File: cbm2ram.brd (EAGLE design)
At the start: 133.3 x 120.7 mm, 21 parts, among them U1 74574N, U2 74574N, U3 GAL16V8, U4 74LS04N, U5 HM628512A_DIL32, U6 HM628512A_DIL32, U7 74541N, U8 74541N

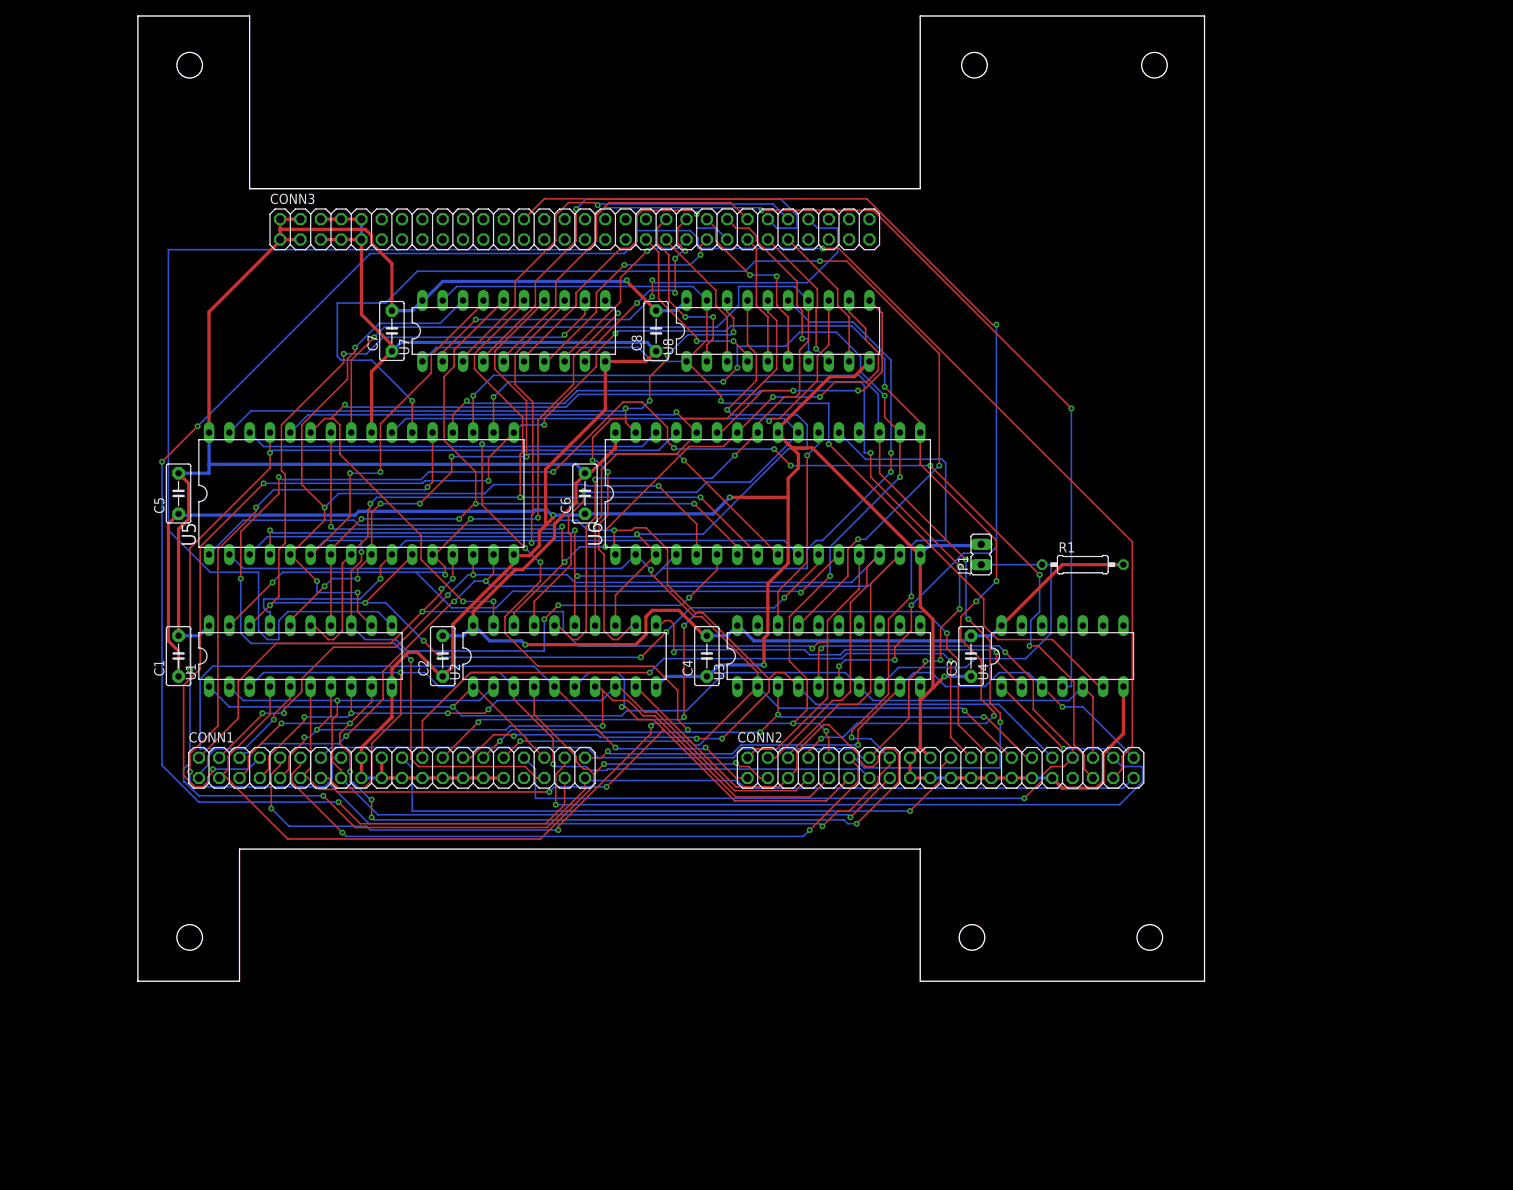
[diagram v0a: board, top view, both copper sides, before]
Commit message: Added EPROM chips
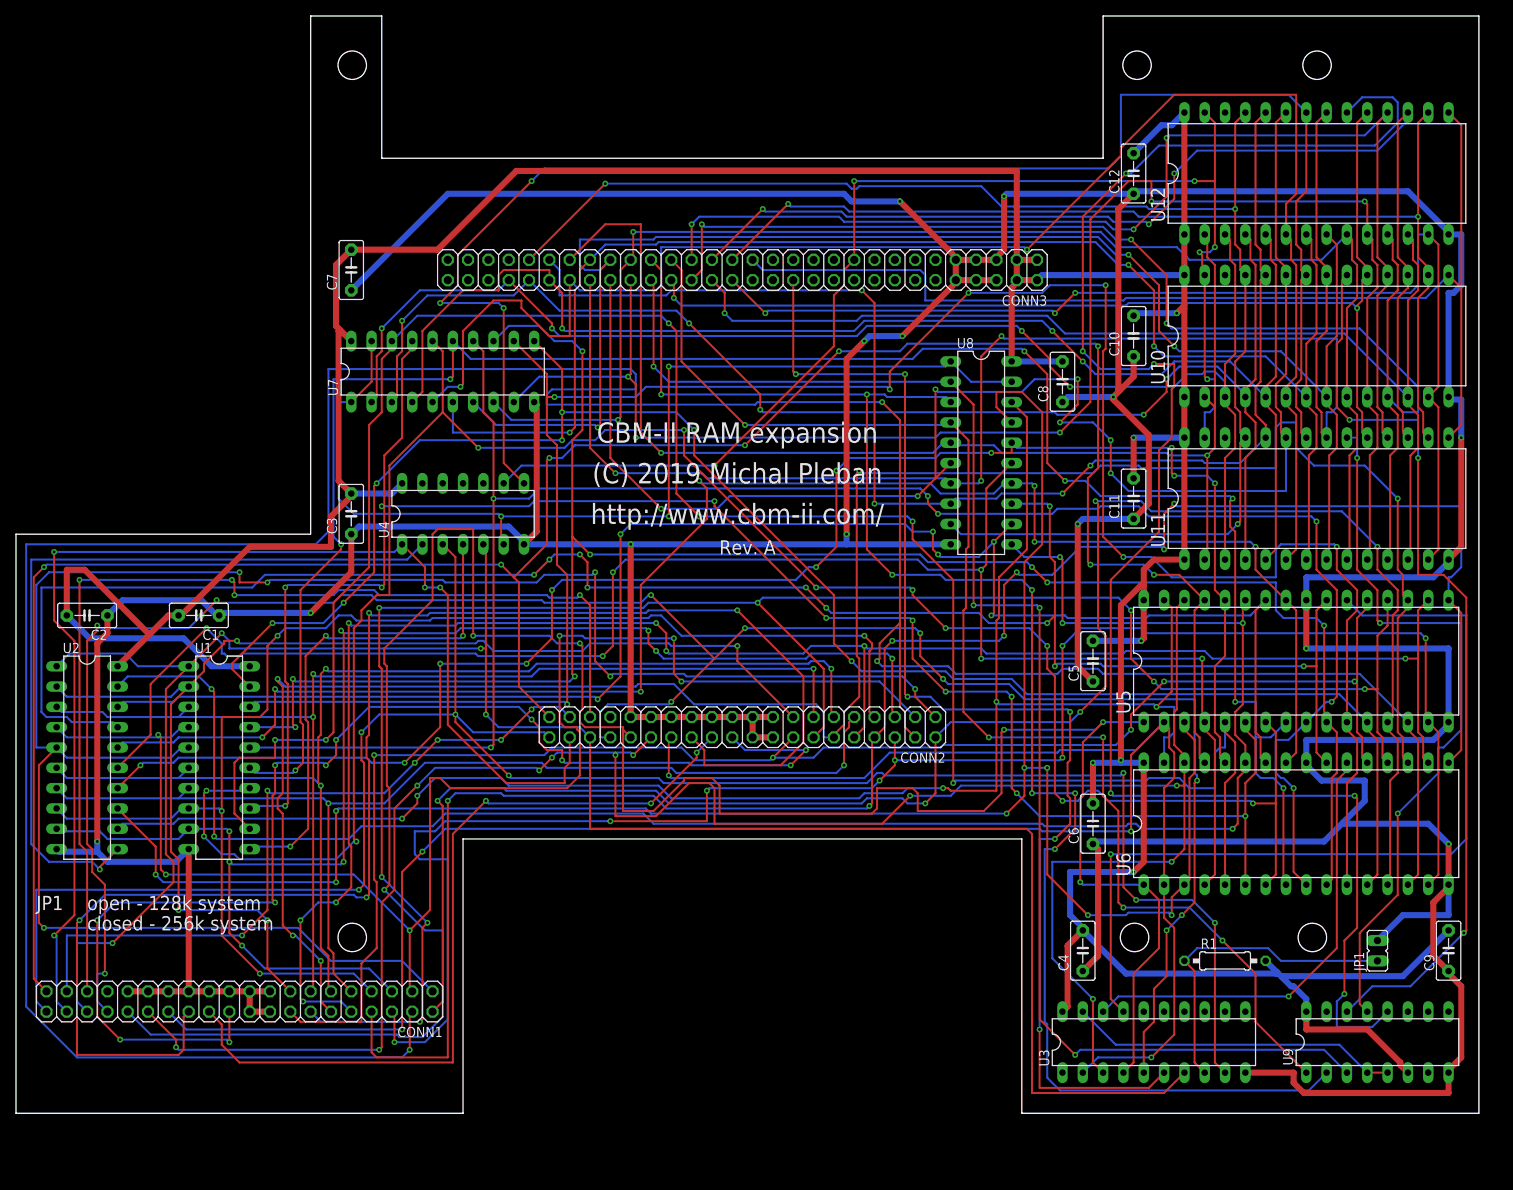
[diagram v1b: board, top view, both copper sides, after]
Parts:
- added C10, C11, C12, C9: 330n, capacitor-wima:C5B3
- added U10, U11, U12: 27C64P, microchip:DIL28-6
- added U9: 74138N, 74ttl-din@1:DIL16
- moved U5 118.7 mm to (143.5, 40.0)
- moved C5 116.2 mm to (119.4, 40.0)
- moved C3 79.5 mm to (26.7, 58.4)
- moved U6 77.9 mm to (143.5, 19.7)
- moved U4 77.0 mm to (40.6, 58.4)
- moved C6 75.7 mm to (119.4, 19.7)
- moved JP1 70.0 mm to (154.9, 3.81)
- moved U3 63.1 mm to (127.0, -7.62)
- moved U2 61.0 mm to (-6.35, 27.9), turned to 270 degrees
- moved C4 59.7 mm to (118.1, 3.81)
- moved R1 52.6 mm to (135.9, 2.54)
- moved C8 51.2 mm to (115.6, 74.9)
- moved C2 44.7 mm to (-6.35, 45.7), turned to 180 degrees
- moved CONN1 34.9 mm to (12.7, -2.54), turned to 180 degrees
- moved U8 29.6 mm to (105.4, 66.0), turned to 270 degrees
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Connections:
- new net /WE: CONN3.19, U10.27, U11.27, U12.27, U4.9
- new net MD0: CONN3.36, U10.11, U11.11, U12.11
- new net MD1: CONN3.34, U10.12, U11.12, U12.12
- new net MD2: CONN3.32, U10.13, U11.13, U12.13
- new net MD3: CONN3.29, U10.15, U11.15, U12.15
- new net MD4: CONN3.31, U10.16, U11.16, U12.16
- new net MD5: CONN3.33, U10.17, U11.17, U12.17
- new net MD6: CONN3.35, U10.18, U11.18, U12.18
- new net MD7: CONN3.38, U10.19, U11.19, U12.19
- new net N$2: U12.20, U9.12
- new net N$3: U11.20, U9.13
- new net N$5: U10.20, U9.14
- new net N$8: U10.22, U11.22, U12.22, U4.8
- net A0: now also U10.10, U11.10, U12.10
- net A1: now also U10.9, U11.9, U12.9
- net A10: now also U10.21, U11.21, U12.21
- net A11: now also U10.23, U11.23, U12.23
- net A12: now also U10.2, U11.2, U12.2
- net A13: now also U9.1
- net A14: now also U9.2
- net A15: now also U9.3
- net A2: now also U10.8, U11.8, U12.8
- net A3: now also U10.7, U11.7, U12.7
- net A4: now also U10.6, U11.6, U12.6
- net A5: now also U10.5, U11.5, U12.5
- net A6: now also U10.4, U11.4, U12.4
- net A7: now also U10.3, U11.3, U12.3
- net A8: now also U10.25, U11.25, U12.25
- net A9: now also U10.24, U11.24, U12.24
- net BANK15: now also U9.4, U9.5
- net GND: now also C10.1, C11.1, C12.1, C9.1, U10.14, U11.14, U12.14, U9.8
- net VCC: now also C10.2, C11.2, C12.2, C9.2, U10.1, U10.28, U11.1, U11.28, U12.1, U12.28, U9.16, U9.6
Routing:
- net GND: track 442.2 -> 831.0 mm, vias 4 -> 13
- net D1: track 130.1 -> 408.7 mm, vias 4 -> 3
- net VCC: track 308.9 -> 523.3 mm, vias 2 -> 6
- net N$2: track 0.00 -> 208.4 mm, vias 0 -> 6
- net N$8: track 0.00 -> 200.6 mm, vias 0 -> 3
- net R/W: track 277.0 -> 91.2 mm, vias 4 -> 6
- net A14: track 18.4 -> 201.4 mm, vias 0 -> 7
- net /ECAS: track 80.3 -> 258.9 mm, vias 3 -> 7
- net ECAS: track 240.0 -> 62.5 mm, vias 2 -> 3
- net A0: track 26.3 -> 203.2 mm, vias 4 -> 5
- net SA5: track 96.1 -> 262.4 mm, vias 4 -> 11
- net A8: track 18.4 -> 184.7 mm, vias 0 -> 3
- net A10: track 23.4 -> 189.0 mm, vias 1 -> 3
- net A11: track 23.8 -> 189.4 mm, vias 2 -> 7
- net A2: track 28.7 -> 194.1 mm, vias 2 -> 3
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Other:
- board size 133.3 x 120.7 mm -> 182.9 x 137.2 mm
- board text added: "(C) 2019 Michal Pleban"
- board text added: "CBM-II RAM expansion"
- board text added: "JP1"
- board text added: "Rev. A"
- board text added: "closed - 256k system"
- board text added: "http://www.cbm-ii.com/"
- board text added: "open - 128k system"

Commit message: Complete board.
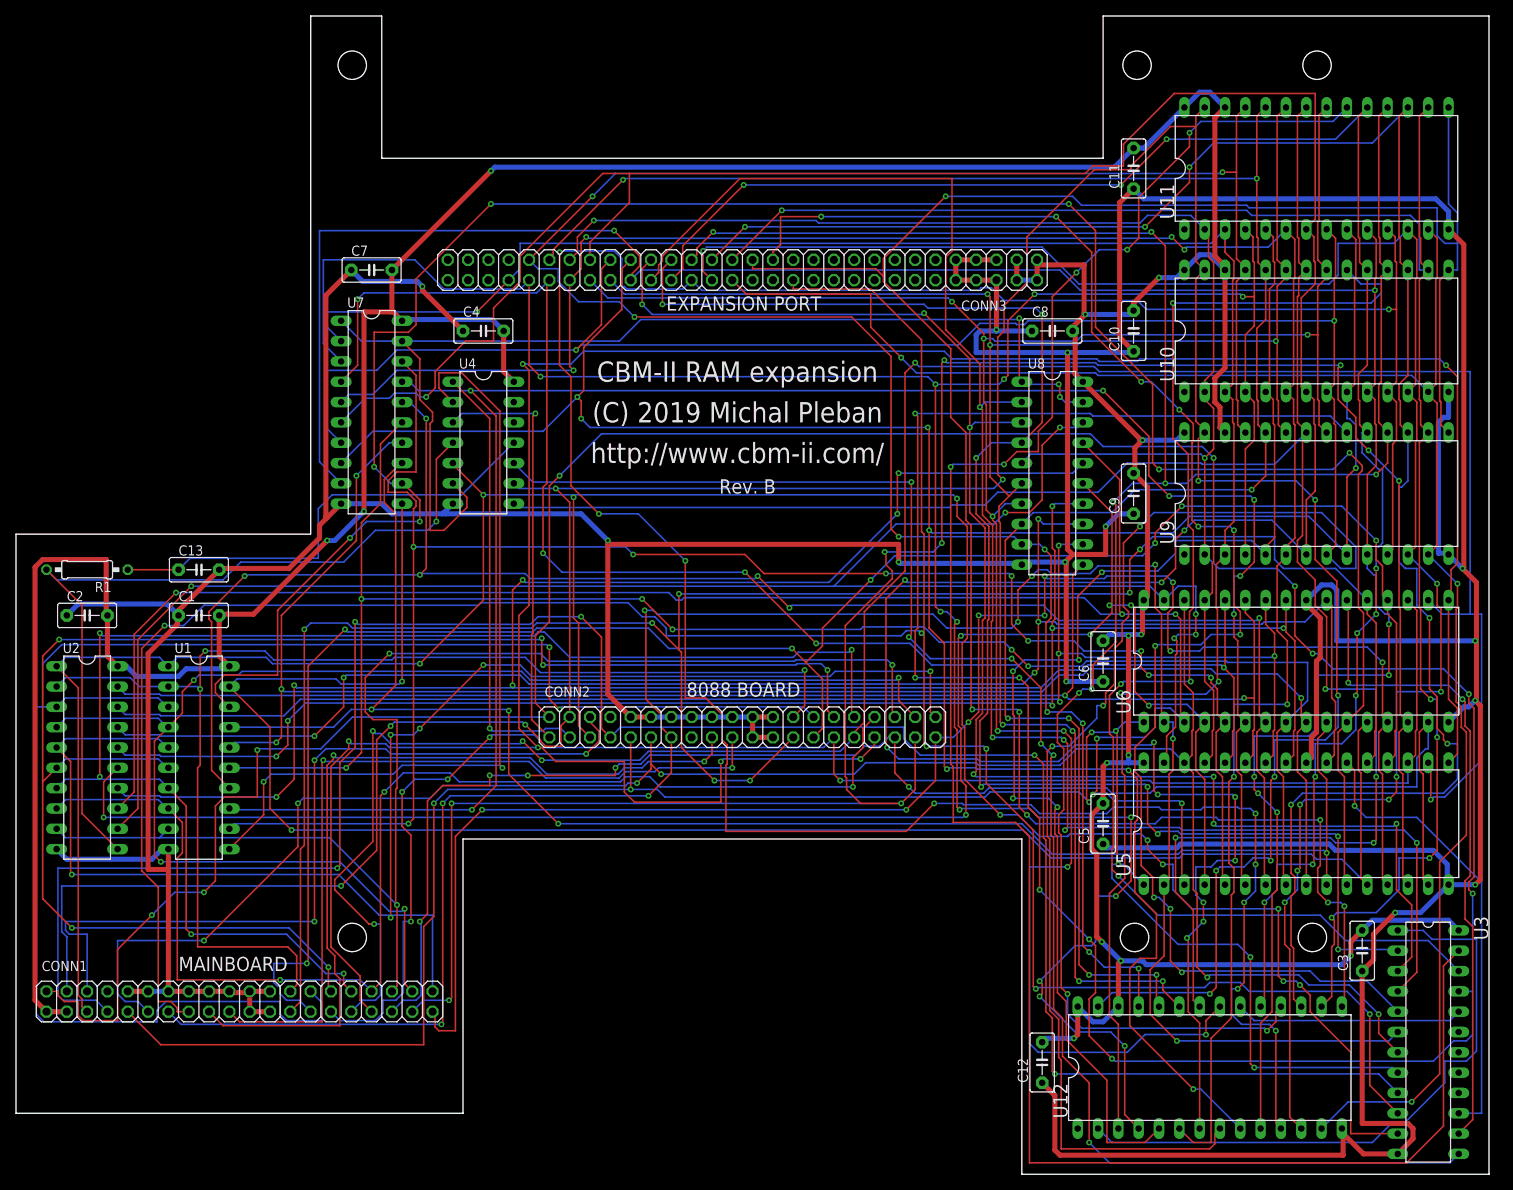
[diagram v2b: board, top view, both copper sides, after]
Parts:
- removed JP1: (no value), jumper:JP1
- added C13: 220n, capacitor-wima:C5B3
- R1: value 5.1k -> 1k
- U10, U11, U12: value 27C64P -> (none); device microchip:DIL28-6 -> memory-hitachi:DIL28-6
- U3: value GAL16V8 -> (none); device pal:DIL20 -> pal:DIL24-3
- U9: value 74138N -> (none); device 74ttl-din@1:DIL16 -> memory-hitachi:DIL28-6
- moved R1 150.4 mm to (-6.35, 51.4), turned to 180 degrees
- moved C3 137.7 mm to (153.0, 3.81)
- moved U12 112.6 mm to (134.0, -10.8)
- moved C12 111.7 mm to (113.0, -10.2)
- moved C4 107.8 mm to (43.2, 81.3), turned to 0 degrees
- moved C9 69.4 mm to (124.5, 61.0)
- moved U9 69.0 mm to (147.3, 61.0)
- moved C11 41.3 mm to (124.5, 101.6)
- moved U11 41.3 mm to (147.3, 101.6)
- moved U3 34.3 mm to (161.3, -7.62), turned to 270 degrees
- moved C5 20.4 mm to (120.7, 19.7)
- moved C6 20.4 mm to (120.7, 40.0)
- moved U5 20.3 mm to (143.5, 19.7)
- moved U6 20.3 mm to (143.5, 40.0)
- moved U7 10.2 mm to (29.2, 71.1), turned to 270 degrees
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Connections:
- removed net /P2REFGNT: CONN1.26, CONN2.26
- removed net /WE: CONN3.19, U10.27, U11.27, U12.27, U4.9
- removed net BANK15: U3.19, U9.4, U9.5
- removed net N$1: JP1.1, R1.1, U3.8
- removed net N$2: U12.20, U9.12
- removed net N$3: U11.20, U9.13
- removed net N$5: U10.20, U9.14
- removed net N$8: U10.22, U11.22, U12.22, U4.8
- new net /ECAS': U3.13, U4.10
- new net /OE: U10.22, U11.22, U12.22, U4.8, U9.22
- new net /RAM1: U12.20, U3.20
- new net /ROM1: U3.21, U9.20
- new net /ROM2: U10.20, U3.22
- new net /ROM3: U11.20, U3.23
- new net ECAS': C13.1, R1.1, U4.11
- new net PHI1: CONN3.27, U3.5
- net /BUSY2: now also U3.11; no longer U3.7
- net /CAS: now also CONN1.26, U3.10; no longer U3.6
- net /CS1: now also U3.15; no longer U3.17
- net /CS2: now also U3.14; no longer U3.18
- net /ECAS: no longer CONN1.40, U3.9
- net /ERAS: no longer CONN1.38
- net A0: now also U9.10
- net A1: now also U9.9
- net A10: now also U9.21
- net A11: now also U9.23
- net A12: now also U3.1, U9.2
- net A13: now also U3.2; no longer U9.1
- net A14: now also U3.3; no longer U9.2
- net A15: now also U3.4; no longer U9.3
- net A2: now also U9.8
- net A3: now also U9.7
- net A4: now also U9.6
- net A5: now also U9.5
- net A6: now also U9.4
- net A7: now also U9.3
- net A8: now also U9.25
- net A9: now also U9.24
- net BP0: now also U3.6; no longer U3.2
- net BP1: now also U3.7; no longer U3.3
- net BP2: now also U3.8; no longer U3.4
- net BP3: now also U3.9; no longer U3.5
- net ECAS: now also R1.2, U2.11; no longer U1.11
- net ERAS: now also U1.11; no longer U2.11
- net GND: now also C13.2, U3.12, U9.14; no longer JP1.2, U3.10, U9.8
- net MD0: now also U9.11
- net MD1: now also U9.12
- net MD2: now also U9.13
- net MD3: now also U9.15
- net MD4: now also U9.16
- net MD5: now also U9.17
- net MD6: now also U9.18
- net MD7: now also U9.19
- net R/W: now also U10.27, U11.27, U12.27, U4.9, U9.27
- net VCC: now also CONN1.38, CONN1.40, U10.26, U11.26, U12.26, U3.24, U9.26, U9.28; no longer R1.2, U10.1, U11.1, U12.1, U3.20, U9.16, U9.6
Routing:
- net R/W: track 91.2 -> 404.2 mm, vias 6 -> 12
- net /ROM3: track 0.00 -> 254.4 mm, vias 0 -> 5
- net /OE: track 0.00 -> 252.9 mm, vias 0 -> 4
- net A3: track 186.4 -> 398.3 mm, vias 3 -> 12
- net N$2: track 208.4 -> 0.00 mm, vias 6 -> 0
- net /ROM1: track 0.00 -> 208.1 mm, vias 0 -> 6
- net /ECAS: track 258.9 -> 52.4 mm, vias 7 -> 1
- net N$8: track 200.6 -> 0.00 mm, vias 3 -> 0
- net /ECAS': track 0.00 -> 196.7 mm, vias 0 -> 6
- net MD0: track 159.5 -> 353.7 mm, vias 3 -> 10
- net /P2REFGNT: track 192.9 -> 0.00 mm, vias 4 -> 0
- net PHI1: track 0.00 -> 190.2 mm, vias 0 -> 11
- net /CAS: track 153.4 -> 321.0 mm
- net /ROM2: track 0.00 -> 162.8 mm, vias 0 -> 4
- net /WE: track 160.1 -> 0.00 mm, vias 6 -> 0
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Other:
- board size 182.9 x 137.2 mm -> 184.1 x 144.8 mm
- board text added: "8088 BOARD"
- board text added: "EXPANSION PORT"
- board text added: "MAINBOARD"
- board text added: "Rev. B"
- board text removed: "JP1"
- board text removed: "Rev. A"
- board text removed: "closed - 256k system"
- board text removed: "open - 128k system"
